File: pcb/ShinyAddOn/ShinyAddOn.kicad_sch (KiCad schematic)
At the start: 3 parts, among them J1 Conn_02x03_Odd_Even

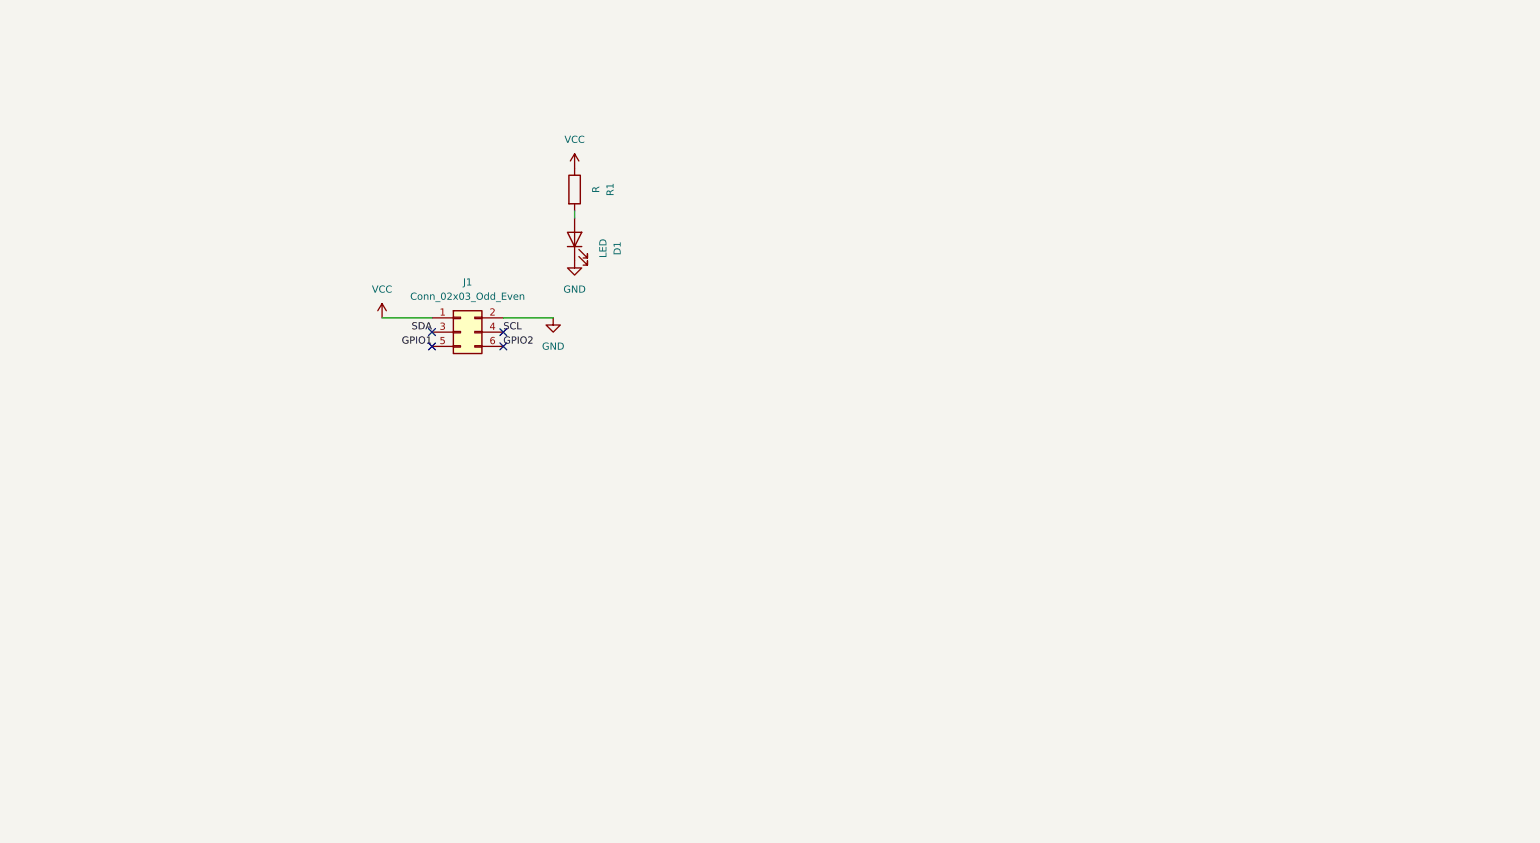
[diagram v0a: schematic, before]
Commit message: worked on the pcb
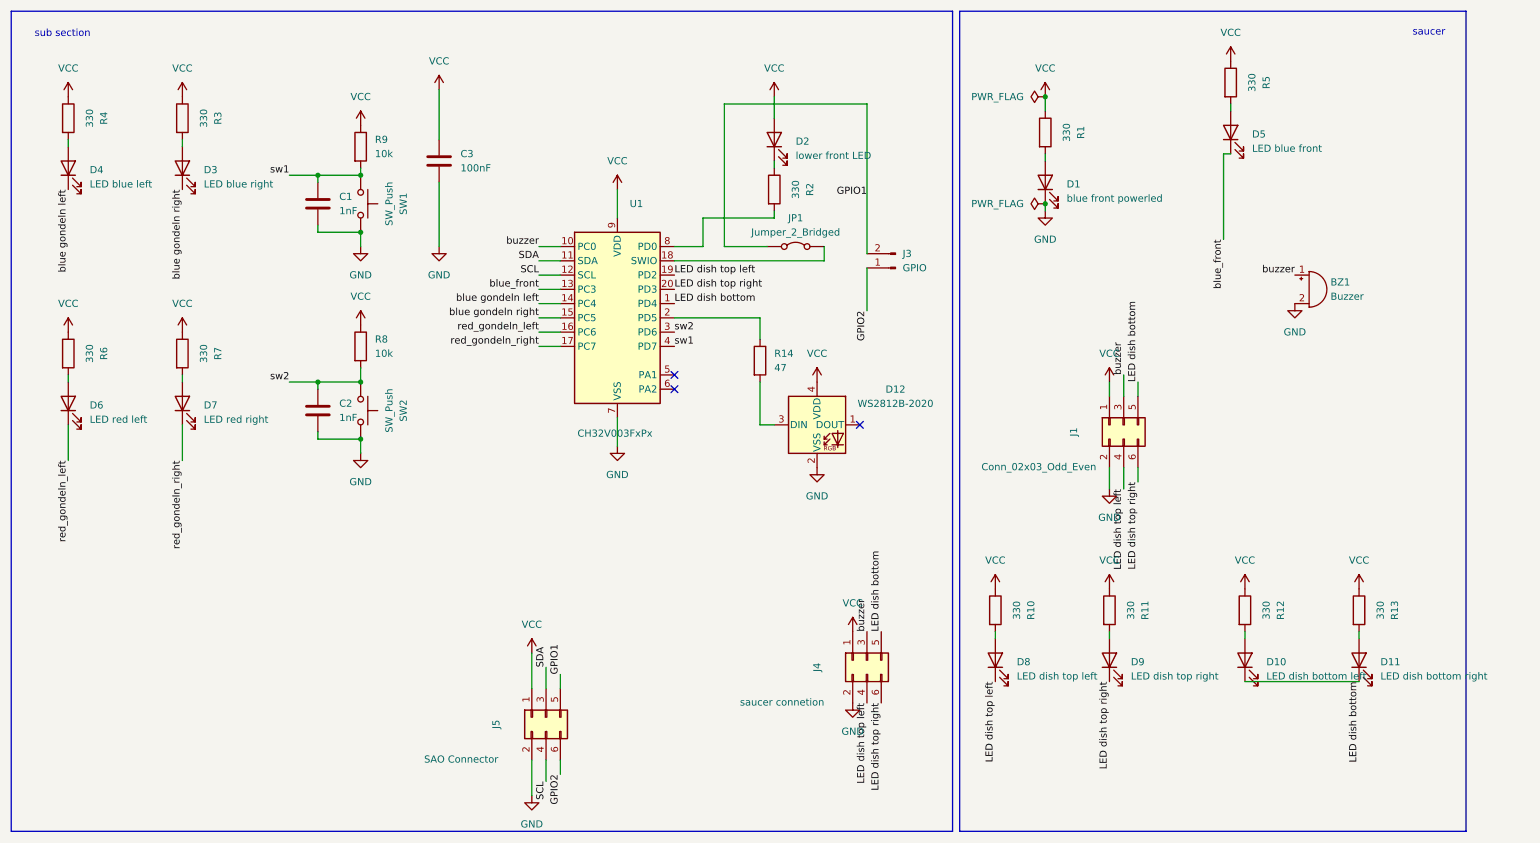
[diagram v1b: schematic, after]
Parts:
- added BZ1: Buzzer, Buzzer_Beeper:Buzzer_12x9.5RM7.6, symbol Device:Buzzer
- added C1, C2: 1nF, Capacitor_SMD:C_0603_1608Metric_Pad1.08x0.95mm_HandSolder, symbol Device:C
- added C3: 100nF, Capacitor_SMD:C_0603_1608Metric_Pad1.08x0.95mm_HandSolder, symbol Device:C
- added D10: LED dish bottom left, LED_SMD:LED_0603_1608Metric_Pad1.05x0.95mm_HandSolder, symbol Device:LED
- added D11: LED dish bottom right, LED_SMD:LED_0603_1608Metric_Pad1.05x0.95mm_HandSolder, symbol Device:LED
- added D12: WS2812B-2020, LED_SMD:LED_WS2812B-2020_PLCC4_2.0x2.0mm, symbol LED:WS2812B-2020
- added D2: lower front LED, LED_SMD:LED_0603_1608Metric_Pad1.05x0.95mm_HandSolder, symbol Device:LED
- added D3: LED blue right, LED_SMD:LED_0603_1608Metric_Pad1.05x0.95mm_HandSolder, symbol Device:LED
- added D4: LED blue left, LED_SMD:LED_0603_1608Metric_Pad1.05x0.95mm_HandSolder, symbol Device:LED
- added D5: LED blue front, LED_SMD:LED_0603_1608Metric_Pad1.05x0.95mm_HandSolder, symbol Device:LED
- added D6: LED red left, LED_SMD:LED_0603_1608Metric_Pad1.05x0.95mm_HandSolder, symbol Device:LED
- added D7: LED red right, LED_SMD:LED_0603_1608Metric_Pad1.05x0.95mm_HandSolder, symbol Device:LED
- added D8: LED dish top left, LED_SMD:LED_0603_1608Metric_Pad1.05x0.95mm_HandSolder, symbol Device:LED
- added D9: LED dish top right, LED_SMD:LED_0603_1608Metric_Pad1.05x0.95mm_HandSolder, symbol Device:LED
- added J3: GPIO, Jumper:SolderJumper-2_P1.3mm_Open_RoundedPad1.0x1.5mm, symbol Connector:Conn_01x02_Pin
- added J4: saucer connetion, Connector_PinSocket_2.54mm:PinSocket_2x03_P2.54mm_Vertical, symbol Connector_Generic:Conn_02x03_Odd_Even
- added J5: SAO Connector, Connector_PinHeader_2.54mm:PinHeader_2x03_P2.54mm_Vertical, symbol Connector_Generic:Conn_02x03_Odd_Even
- added JP1: Jumper_2_Bridged, Jumper:SolderJumper-2_P1.3mm_Bridged_RoundedPad1.0x1.5mm, symbol Jumper:Jumper_2_Bridged
- added R10, R11, R12, R13, R2, R3, R4, R5, R6, R7: 330, Resistor_SMD:R_0603_1608Metric_Pad0.98x0.95mm_HandSolder, symbol Device:R
- added R14: 47, Resistor_SMD:R_0603_1608Metric_Pad0.98x0.95mm_HandSolder, symbol Device:R
- added R8, R9: 10k, Resistor_SMD:R_0603_1608Metric_Pad0.98x0.95mm_HandSolder, symbol Device:R
- added SW1, SW2: SW_Push, Button_Switch_SMD:SW_Tactile_SPST_NO_Straight_CK_PTS636Sx25SMTRLFS, symbol Switch:SW_Push
- added U1: CH32V003FxPx, Package_SO:TSSOP-20_4.4x6.5mm_P0.65mm, symbol MCU_WCH_CH32V0:CH32V003FxPx
- D1: value LED -> blue front powerled; footprint LED_SMD:LED_0805_2012Metric_Pad1.15x1.40mm_HandSolder -> LED_SMD:LED_0603_1608Metric_Pad1.05x0.95mm_HandSolder
- R1: value R -> 330; footprint Resistor_SMD:R_0805_2012Metric_Pad1.20x1.40mm_HandSolder -> Resistor_SMD:R_0603_1608Metric_Pad0.98x0.95mm_HandSolder
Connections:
- net GND: now also BZ1.2 (-), C1.2, C2.2, C3.2, D12.2 (VSS), J4.2 (Pin_2), J5.2 (Pin_2), SW1.2, SW2.2, U1.7 (VSS)
- net GPIO1: now also J3.2 (Pin_2), J5.5 (Pin_5), JP1.1 (A); no longer J1.5 (Pin_5)
- net GPIO2: now also J3.1 (Pin_1), J5.6 (Pin_6); no longer J1.6 (Pin_6)
- net SCL: now also J5.4 (Pin_4), U1.12 (PC2); no longer J1.4 (Pin_4)
- net SDA: now also J5.3 (Pin_3), U1.11 (PC1); no longer J1.3 (Pin_3)
- net VCC: now also C3.1, D12.4 (VDD), D2.2 (A), J4.1 (Pin_1), J5.1 (Pin_1), R10.1, R11.1, R12.1, R13.1, R3.1, R4.1, R5.1, R6.1, R7.1, R8.1, R9.1, U1.9 (VDD)
- new net: D11.2 (A), R13.2
- new net: D2.1 (K), R2.1
- new net: R2.2, U1.8 (PD0)
- new net: D3.2 (A), R3.2
- new net: R14.1, U1.2 (PD5)
- new net: D12.3 (DIN), R14.2
- new net: D6.2 (A), R6.2
- new net: D4.2 (A), R4.2
- new net: D5.2 (A), R5.2
- new net: D7.2 (A), R7.2
- new net: JP1.2 (B), U1.18 (PD1)
- new net: D10.2 (A), R12.2
- new net: D9.2 (A), R11.2
- new net: D8.2 (A), R10.2
- new net LED dish bottom: D10.1 (K), D11.1 (K), J1.5 (Pin_5), J4.5 (Pin_5), U1.1 (PD4)
- new net LED dish top left: D8.1 (K), J1.4 (Pin_4), J4.4 (Pin_4), U1.19 (PD2)
- new net LED dish top right: D9.1 (K), J1.6 (Pin_6), J4.6 (Pin_6), U1.20 (PD3)
- new net blue gondeln left: D4.1 (K), U1.14 (PC4)
- new net blue gondeln right: D3.1 (K), U1.15 (PC5)
- new net blue_front: D5.1 (K), U1.13 (PC3)
- new net buzzer: BZ1.1 (+), J1.3 (Pin_3), J4.3 (Pin_3), U1.10 (PC0)
- new net red_gondeln_left: D6.1 (K), U1.16 (PC6)
- new net red_gondeln_right: D7.1 (K), U1.17 (PC7)
- new net sw1: C1.1, R9.2, SW1.1, U1.4 (PD7)
- new net sw2: C2.1, R8.2, SW2.1, U1.3 (PD6)
- no-connect marks 4 -> 3
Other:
- note added: "saucer"
- note added: "sub section"
- moved on the sheet: D1, J1, R1
